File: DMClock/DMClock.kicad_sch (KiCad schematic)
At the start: 4 parts, among them J5 Conn_01x07_Pin, J6 Conn_01x07_Pin, J7 Conn_01x07_Pin, J8 Conn_01x07_Pin

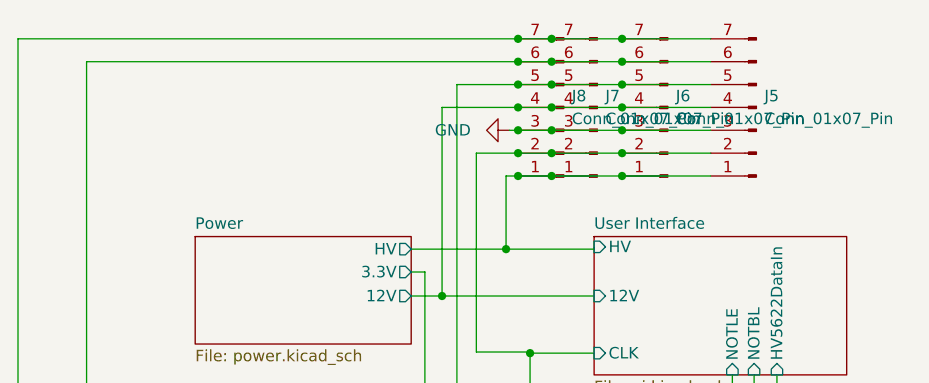
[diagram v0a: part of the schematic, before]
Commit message: update second layer finalizations
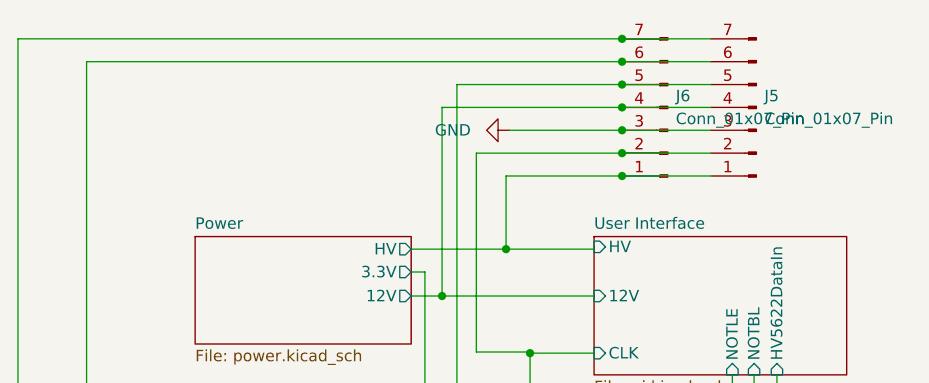
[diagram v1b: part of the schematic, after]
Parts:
- removed J7, J8: Conn_01x07_Pin, Connector_PinSocket_2.54mm:PinSocket_1x07_P2.54mm_Vertical, symbol Connector:Conn_01x07_Pin
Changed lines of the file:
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@@
   (junction (at 123.6883 77.597) (diameter 0) (color 0 0 0 0)
   )
-  (junction (at 108.1415 41.402) (diameter 0) (color 0 0 0 0)
-  )
-  (junction (at 108.1415 33.782) (diameter 0) (color 0 0 0 0)
-  )
   (junction (at 109.474 61.087) (diameter 0) (color 0 0 0 0)
   )
-  (junction (at 108.1415 26.162) (diameter 0) (color 0 0 0 0)
-  )
   (junction (at 119.6963 33.782) (diameter 0) (color 0 0 0 0)
   )
-  (junction (at 108.1415 31.242) (diameter 0) (color 0 0 0 0)
-  )
   (junction (at 123.317 81.407) (diameter 0) (color 0 0 0 0)
   )
   (junction (at 119.6963 41.402) (diameter 0) (color 0 0 0 0)
   )
-  (junction (at 111.8702 28.702) (diameter 0) (color 0 0 0 0)
-  )
-  (junction (at 111.8702 31.242) (diameter 0) (color 0 0 0 0)
-  )
-  (junction (at 111.8702 36.322) (diameter 0) (color 0 0 0 0)
-  )
   (junction (at 125.349 79.502) (diameter 0) (color 0 0 0 0)
   )
   (junction (at 119.6963 26.162) (diameter 0) (color 0 0 0 0)
   )
-  (junction (at 108.1415 36.322) (diameter 0) (color 0 0 0 0)
-  )
-  (junction (at 111.8702 41.402) (diameter 0) (color 0 0 0 0)
-  )
   (junction (at 119.6963 28.702) (diameter 0) (color 0 0 0 0)
   )
   (junction (at 119.6963 38.862) (diameter 0) (color 0 0 0 0)
   )
-  (junction (at 108.1415 38.862) (diameter 0) (color 0 0 0 0)
-  )
   (junction (at 119.6963 31.242) (diameter 0) (color 0 0 0 0)
   )
   (junction (at 99.695 54.737) (diameter 0) (color 0 0 0 0)
   )
-  (junction (at 111.8702 33.782) (diameter 0) (color 0 0 0 0)
-  )
-  (junction (at 108.1415 28.702) (diameter 0) (color 0 0 0 0)
-  )
-  (junction (at 111.8702 26.162) (diameter 0) (color 0 0 0 0)
-  )
-  (junction (at 111.8702 38.862) (diameter 0) (color 0 0 0 0)
-  )
   (junction (at 106.807 49.53) (diameter 0) (color 0 0 0 0)
   )
@@
     (stroke (width 0) (type default))
   )
-  (wire (pts (xy 108.1415 26.162) (xy 111.8702 26.162))
-    (stroke (width 0) (type default))
-  )
   (wire (pts (xy 125.349 79.502) (xy 125.349 119.126))
     (stroke (width 0) (type default))
@@
     (stroke (width 0) (type default))
   )
-  (wire (pts (xy 106.807 41.402) (xy 108.1415 41.402))
-    (stroke (width 0) (type default))
-  )
   (wire (pts (xy 120.777 81.407) (xy 123.317 81.407))
     (stroke (width 0) (type default))
@@
     (stroke (width 0) (type default))
   )
-  (wire (pts (xy 111.8702 26.162) (xy 119.6963 26.162))
+  (wire (pts (xy 52.578 26.162) (xy 119.6963 26.162))
     (stroke (width 0) (type default))
   )
@@
     (stroke (width 0) (type default))
   )
-  (wire (pts (xy 52.578 26.162) (xy 108.1415 26.162))
-    (stroke (width 0) (type default))
-  )
-  (wire (pts (xy 111.8702 28.702) (xy 119.6963 28.702))
-    (stroke (width 0) (type default))
-  )
-  (wire (pts (xy 111.8702 31.242) (xy 119.6963 31.242))
-    (stroke (width 0) (type default))
-  )
-  (wire (pts (xy 99.695 33.782) (xy 108.1415 33.782))
+  (wire (pts (xy 99.695 33.782) (xy 119.6963 33.782))
     (stroke (width 0) (type default))
   )
@@
     (stroke (width 0) (type default))
   )
-  (wire (pts (xy 111.8702 38.862) (xy 119.6963 38.862))
-    (stroke (width 0) (type default))
-  )
   (wire (pts (xy 99.695 54.737) (xy 116.586 54.737))
     (stroke (width 0) (type default))
@@
     (stroke (width 0) (type default))
   )
-  (wire (pts (xy 108.1415 38.862) (xy 111.8702 38.862))
+  (wire (pts (xy 103.505 38.862) (xy 119.6963 38.862))
     (stroke (width 0) (type default))
   )
@@
     (stroke (width 0) (type default))
   )
-  (wire (pts (xy 108.1415 36.322) (xy 107.188 36.322))
-    (stroke (width 0) (type default))
-  )
   (wire (pts (xy 106.807 41.402) (xy 106.807 49.53))
     (stroke (width 0) (type default))
   )
-  (wire (pts (xy 108.1415 31.242) (xy 111.8702 31.242))
+  (wire (pts (xy 101.346 31.242) (xy 119.6963 31.242))
     (stroke (width 0) (type default))
   )
@@
     (stroke (width 0) (type default))
   )
-  (wire (pts (xy 60.198 28.702) (xy 108.1415 28.702))
+  (wire (pts (xy 60.198 28.702) (xy 119.6963 28.702))
     (stroke (width 0) (type default))
   )
@@
     (stroke (width 0) (type default))
   )
-  (wire (pts (xy 119.6963 36.322) (xy 111.8702 36.322))
-    (stroke (width 0) (type default))
-  )
   (wire (pts (xy 116.586 49.53) (xy 116.586 49.276))
     (stroke (width 0) (type default))
@@
     (stroke (width 0) (type default))
   )
-  (wire (pts (xy 108.1415 28.702) (xy 111.8702 28.702))
-    (stroke (width 0) (type default))
-  )
   (wire (pts (xy 106.807 49.53) (xy 116.586 49.53))
     (stroke (width 0) (type default))
   )
-  (wire (pts (xy 111.8702 36.322) (xy 108.1415 36.322))
+  (wire (pts (xy 107.188 36.322) (xy 119.6963 36.322))
     (stroke (width 0) (type default))
   )
@@
     (stroke (width 0) (type default))
   )
-  (wire (pts (xy 108.1415 41.402) (xy 111.8702 41.402))
+  (wire (pts (xy 106.807 41.402) (xy 119.6963 41.402))
     (stroke (width 0) (type default))
   )
@@
     (stroke (width 0) (type default))
   )
-  (wire (pts (xy 101.346 31.242) (xy 108.1415 31.242))
-    (stroke (width 0) (type default))
-  )
-  (wire (pts (xy 108.1415 33.782) (xy 111.8702 33.782))
-    (stroke (width 0) (type default))
-  )
   (wire (pts (xy 134.366 79.502) (xy 125.349 79.502))
     (stroke (width 0) (type default))
   )
-  (wire (pts (xy 111.8702 33.782) (xy 119.6963 33.782))
-    (stroke (width 0) (type default))
-  )
   (wire (pts (xy 109.474 60.96) (xy 109.474 61.087))
     (stroke (width 0) (type default))
   )
-  (wire (pts (xy 111.8702 41.402) (xy 119.6963 41.402))
-    (stroke (width 0) (type default))
-  )
   (wire (pts (xy 99.695 54.737) (xy 99.695 33.782))
     (stroke (width 0) (type default))
@@
     (stroke (width 0) (type default))
   )
-  (wire (pts (xy 103.505 38.862) (xy 108.1415 38.862))
-    (stroke (width 0) (type default))
-  )
   (wire (pts (xy 103.505 60.96) (xy 103.505 38.862))
     (stroke (width 0) (type default))
@@
   (wire (pts (xy 119.6963 26.162) (xy 129.54 26.162))
     (stroke (width 0) (type default))
-  )
-  (symbol (lib_id "Connector:Conn_01x07_Pin") (at 113.2215 33.782 180) (unit 1)
-    (in_bom yes) (on_board yes) (dnp no) (fields_autoplaced)
-    (property "Reference" "J8" (at 114.1105 32.512 0)
-      (effects (font (size 1.27 1.27)) (justify right))
-    )
-    (property "Value" "Conn_01x07_Pin" (at 114.1105 35.052 0)
-      (effects (font (size 1.27 1.27)) (justify right))
-    )
-    (property "Footprint" "Connector_PinSocket_2.54mm:PinSocket_1x07_P2.54mm_Vertical" (at 113.2215 33.782 0)
-      (effects (font (size 1.27 1.27)) hide)
-    )
-    (property "Datasheet" "~" (at 113.2215 33.782 0)
-      (effects (font (size 1.27 1.27)) hide)
-    )
-    (pin "7")
-    (pin "3")
-    (pin "1")
-    (pin "2")
-    (pin "4")
-    (pin "5")
-    (pin "6")
-    (instances
-      (project "DMClock"
-        (path "/b42b345f-a3f2-4eff-9109-2f4619119d33"
-          (reference "J8") (unit 1)
-        )
-      )
-    )
   )
   (symbol (lib_id "Connector:Conn_01x07_Pin") (at 134.62 33.782 180) (unit 1)
@@
         )
       )
-    )
-  )
-  (symbol (lib_id "Connector:Conn_01x07_Pin") (at 116.9502 33.782 180) (unit 1)
-    (in_bom yes) (on_board yes) (dnp no) (fields_autoplaced)
-    (property "Reference" "J7" (at 117.8392 32.512 0)
-      (effects (font (size 1.27 1.27)) (justify right))
-    )
-    (property "Value" "Conn_01x07_Pin" (at 117.8392 35.052 0)
-      (effects (font (size 1.27 1.27)) (justify right))
-    )
-    (property "Footprint" "Connector_PinSocket_2.54mm:PinSocket_1x07_P2.54mm_Vertical" (at 116.9502 33.782 0)
-      (effects (font (size 1.27 1.27)) hide)
-    )
-    (property "Datasheet" "~" (at 116.9502 33.782 0)
-      (effects (font (size 1.27 1.27)) hide)
-    )
-    (pin "7")
-    (pin "3")
-    (pin "1")
-    (pin "2")
-    (pin "4")
-    (pin "5")
-    (pin "6")
-    (instances
-      (project "DMClock"
-        (path "/b42b345f-a3f2-4eff-9109-2f4619119d33"
-          (reference "J7") (unit 1)
-        )
-      )
